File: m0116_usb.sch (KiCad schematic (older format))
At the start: 20 parts, among them J1 AVR-ISP-6, J2 USB_B_Mini, U1 ATmega32A-PU, Y1 16Mhz

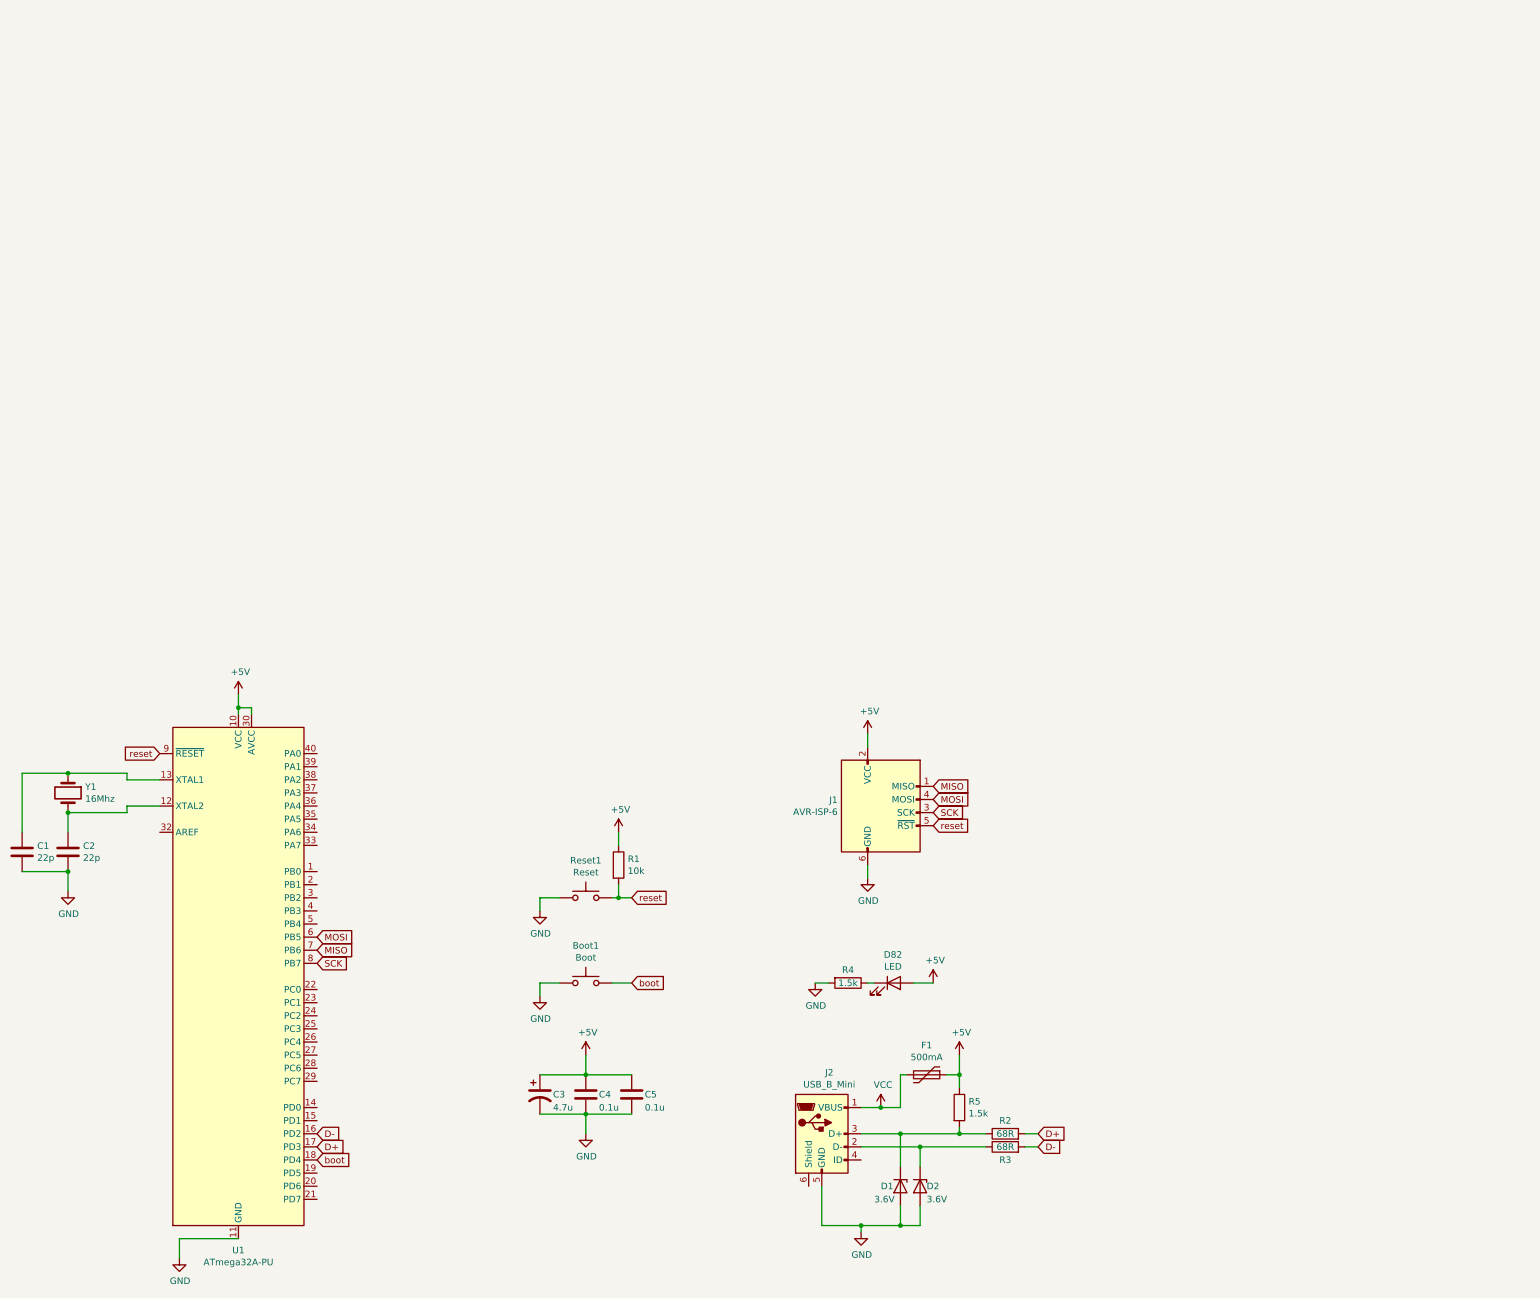
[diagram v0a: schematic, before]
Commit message: finished
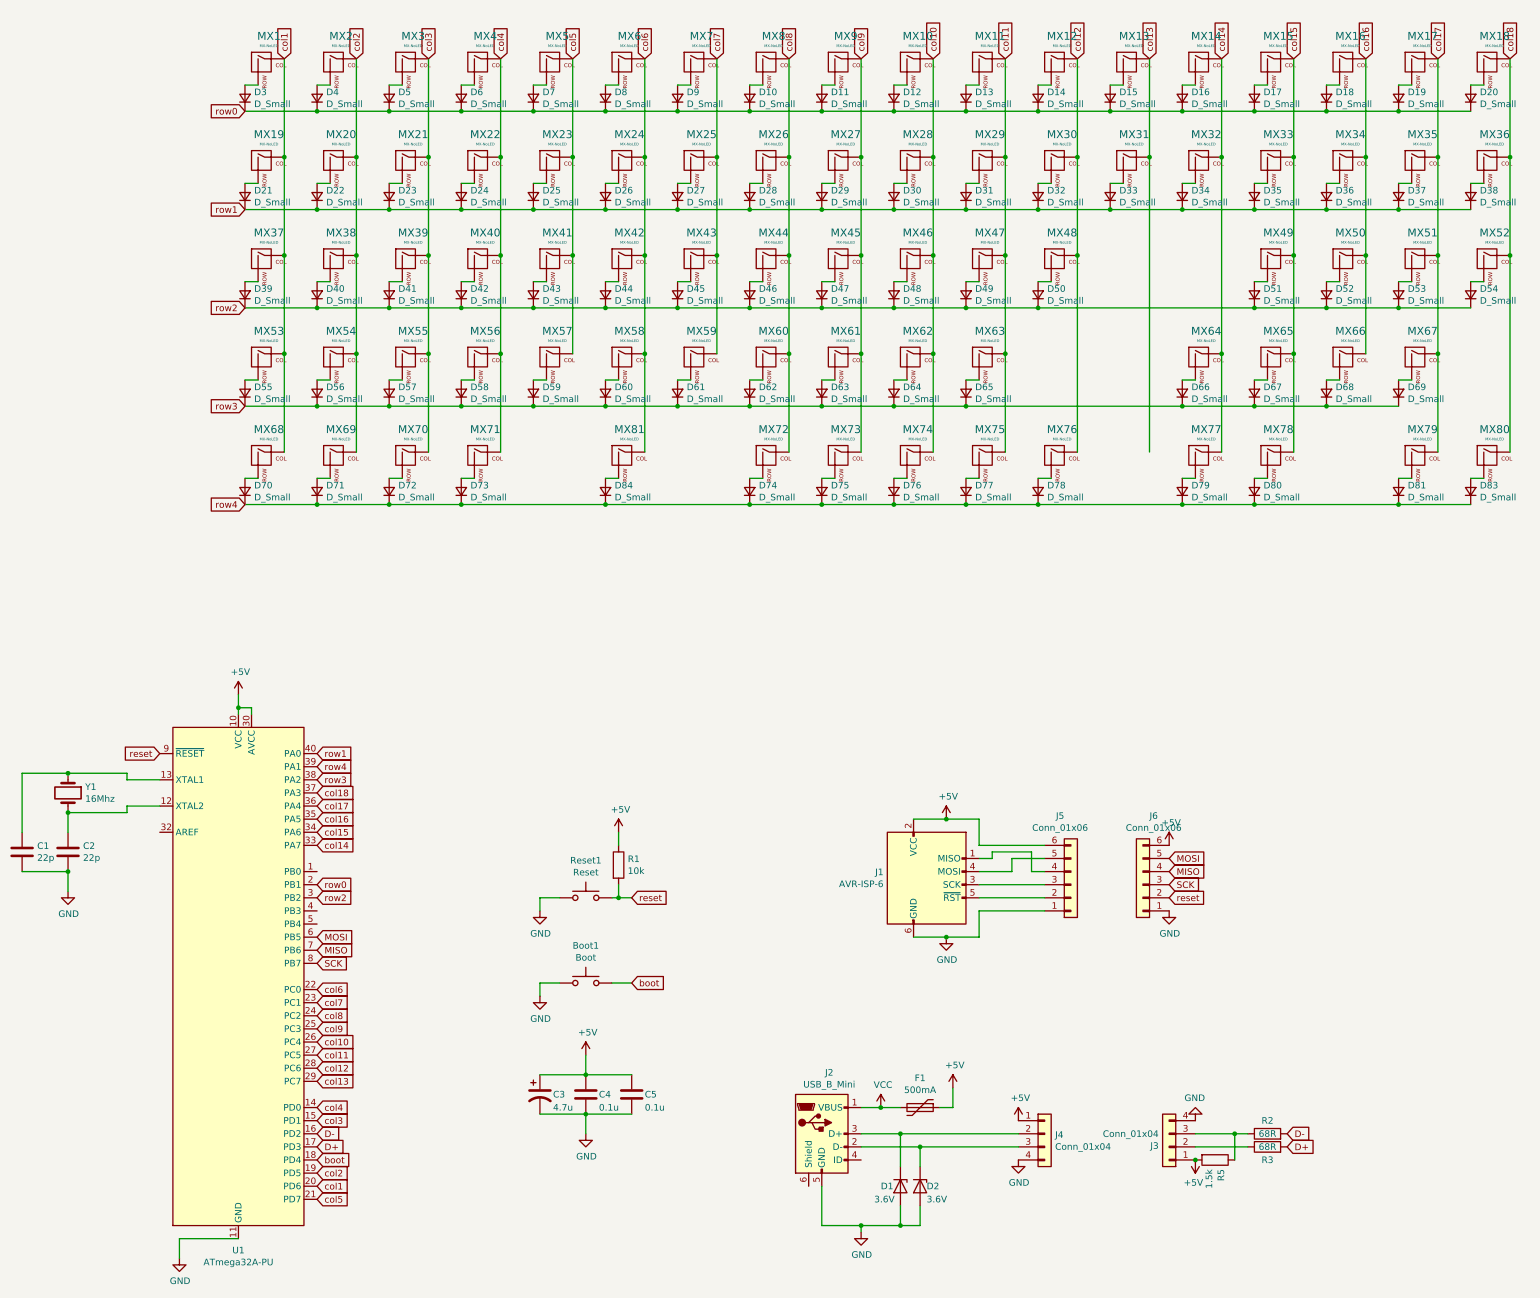
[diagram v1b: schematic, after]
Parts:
- removed D82: LED, LED_THT:LED_D3.0mm, symbol Device:LED
- removed R4: 1.5k, Resistor_THT:R_Axial_DIN0207_L6.3mm_D2.5mm_P10.16mm_Horizontal, symbol Device:R
- added D10, D11, D12, D13, D14, D15, D16, D17, D18, D19, D20, D21, D22, D23, D24, D25, D26, D27, D28, D29, D3, D30, D31, D32, D33, D34, D35, D36, D37, D38, D39, D4, D40, D41, D42, D43, D44, D45, D46, D47, D48, D49, D5, D50, D51, D52, D53, D54, D55, D56, D57, D58, D59, D6, D60, D61, D62, D63, D64, D65, D66, D67, D68, D69, D7, D70, D71, D72, D73, D74, D75, D76, D77, D78, D79, D8, D80, D81, D83, D84, D9: D_Small, Diode_THT:D_DO-35_SOD27_P7.62mm_Horizontal, symbol Device:D_Small
- added J3, J4: Conn_01x04, Connector_PinHeader_2.54mm:PinHeader_1x04_P2.54mm_Vertical, symbol Connector_Generic:Conn_01x04
- added J5, J6: Conn_01x06, Connector_PinHeader_2.54mm:PinHeader_1x06_P2.54mm_Vertical, symbol Connector_Generic:Conn_01x06
- added MX1, MX10, MX11, MX12, MX13, MX14, MX15, MX16, MX17, MX18, MX19, MX2, MX20, MX21, MX22, MX23, MX24, MX25, MX26, MX27, MX28, MX29, MX3, MX30, MX31, MX32, MX33, MX34, MX35, MX36, MX37, MX38, MX39, MX4, MX40, MX41, MX42, MX43, MX44, MX45, MX46, MX47, MX48, MX49, MX5, MX50, MX51, MX52, MX53, MX54, MX55, MX56, MX57, MX58, MX59, MX6, MX60, MX61, MX62, MX63, MX64, MX65, MX66, MX67, MX68, MX69, MX7, MX70, MX71, MX72, MX73, MX74, MX75, MX76, MX77, MX78, MX79, MX8, MX80, MX81, MX9: MX-NoLED, Alps_Only:ALPS-1U, symbol MX_Alps_Hybrid:MX-NoLED
- F1: footprint custom_parts:Fuse_Littelfuse_395Series -> Fuse:Fuse_Littelfuse_395Series
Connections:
- net +5V: now also R5.2, J3.1 (Pin_1), J4.1 (Pin_1), J5.6 (Pin_6), J6.6 (Pin_6); no longer R5.1
- net D+: now also R3.2; no longer R2.2
- net D-: now also R2.2; no longer R3.2
- net GND: now also J3.4 (Pin_4), J4.4 (Pin_4), J5.1 (Pin_1), J6.1 (Pin_1)
- net MISO: now also J6.4 (Pin_4); no longer J1.1 (MISO)
- net MOSI: now also J6.5 (Pin_5); no longer J1.4 (MOSI)
- net SCK: now also J6.3 (Pin_3); no longer J1.3 (SCK)
- net reset: now also J6.2 (Pin_2); no longer J1.5 (~RST)
- net col4: now reaches U1.14 (PD0)
- net col4: now also MX22.1 (COL), MX4.1 (COL), MX40.1 (COL), MX56.1 (COL), MX71.1 (COL)
- net col3: now reaches U1.15 (PD1)
- net col3: now also MX21.1 (COL), MX3.1 (COL), MX39.1 (COL), MX55.1 (COL), MX70.1 (COL)
- net col2: now reaches U1.19 (PD5)
- net col2: now also MX2.1 (COL), MX20.1 (COL), MX38.1 (COL), MX54.1 (COL), MX69.1 (COL)
- net row0: now reaches U1.2 (PB1)
- net row0: now also D10.1 (K), D11.1 (K), D12.1 (K), D13.1 (K), D14.1 (K), D15.1 (K), D16.1 (K), D17.1 (K), D18.1 (K), D19.1 (K), D20.1 (K), D3.1 (K), D4.1 (K), D5.1 (K), D6.1 (K), D7.1 (K), D8.1 (K), D9.1 (K)
- net col1: now reaches U1.20 (PD6)
- net col1: now also MX1.1 (COL), MX19.1 (COL), MX37.1 (COL), MX53.1 (COL), MX68.1 (COL)
- net col5: now reaches U1.21 (PD7)
- net col5: now also MX23.1 (COL), MX41.1 (COL), MX5.1 (COL), MX57.1 (COL)
- net col6: now reaches U1.22 (PC0)
- net col6: now also MX24.1 (COL), MX42.1 (COL), MX58.1 (COL), MX6.1 (COL), MX81.1 (COL)
- net col7: now reaches U1.23 (PC1)
- net col7: now also MX25.1 (COL), MX43.1 (COL), MX59.1 (COL), MX7.1 (COL)
- net col8: now reaches U1.24 (PC2)
- net col8: now also MX26.1 (COL), MX44.1 (COL), MX60.1 (COL), MX72.1 (COL), MX8.1 (COL)
- net col9: now reaches U1.25 (PC3)
- net col9: now also MX27.1 (COL), MX45.1 (COL), MX61.1 (COL), MX73.1 (COL), MX9.1 (COL)
- net col10: now reaches U1.26 (PC4)
- net col10: now also MX10.1 (COL), MX28.1 (COL), MX46.1 (COL), MX62.1 (COL), MX74.1 (COL)
- net col11: now reaches U1.27 (PC5)
- net col11: now also MX11.1 (COL), MX29.1 (COL), MX47.1 (COL), MX63.1 (COL), MX75.1 (COL)
- net col12: now reaches U1.28 (PC6)
- net col12: now also MX12.1 (COL), MX30.1 (COL), MX48.1 (COL), MX76.1 (COL)
- net col13: now reaches U1.29 (PC7)
- net col13: now also MX13.1 (COL), MX31.1 (COL)
- net row2: now reaches U1.3 (PB2)
- net row2: now also D39.1 (K), D40.1 (K), D41.1 (K), D42.1 (K), D43.1 (K), D44.1 (K), D45.1 (K), D46.1 (K), D47.1 (K), D48.1 (K), D49.1 (K), D50.1 (K), D51.1 (K), D52.1 (K), D53.1 (K), D54.1 (K)
- net col14: now reaches U1.33 (PA7)
- net col14: now also MX14.1 (COL), MX32.1 (COL), MX64.1 (COL), MX77.1 (COL)
- net col15: now reaches U1.34 (PA6)
- net col15: now also MX15.1 (COL), MX33.1 (COL), MX49.1 (COL), MX65.1 (COL), MX78.1 (COL)
- net col16: now reaches U1.35 (PA5)
- net col16: now also MX16.1 (COL), MX34.1 (COL), MX50.1 (COL), MX66.1 (COL)
- net col17: now reaches U1.36 (PA4)
- net col17: now also MX17.1 (COL), MX35.1 (COL), MX51.1 (COL), MX67.1 (COL), MX79.1 (COL)
- net col18: now reaches U1.37 (PA3)
- net col18: now also MX18.1 (COL), MX36.1 (COL), MX52.1 (COL), MX80.1 (COL)
- net row3: now reaches U1.38 (PA2)
- net row3: now also D55.1 (K), D56.1 (K), D57.1 (K), D58.1 (K), D59.1 (K), D60.1 (K), D61.1 (K), D62.1 (K), D63.1 (K), D64.1 (K), D65.1 (K), D66.1 (K), D67.1 (K), D68.1 (K), D69.1 (K)
- net row4: now reaches U1.39 (PA1)
- net row4: now also D70.1 (K), D71.1 (K), D72.1 (K), D73.1 (K), D74.1 (K), D75.1 (K), D76.1 (K), D77.1 (K), D78.1 (K), D79.1 (K), D80.1 (K), D81.1 (K), D83.1 (K), D84.1 (K)
- net row1: now reaches U1.40 (PA0)
- net row1: now also D21.1 (K), D22.1 (K), D23.1 (K), D24.1 (K), D25.1 (K), D26.1 (K), D27.1 (K), D28.1 (K), D29.1 (K), D30.1 (K), D31.1 (K), D32.1 (K), D33.1 (K), D34.1 (K), D35.1 (K), D36.1 (K), D37.1 (K), D38.1 (K)
- net at D2.1 (K), J2.2 (D-): now also J4.3 (Pin_3); no longer R3.1
- net at D1.1 (K), J2.3 (D+): now also J4.2 (Pin_2); no longer R2.1, R5.2
- new net: J3.2 (Pin_2), R3.1
- new net: J3.3 (Pin_3), R2.1, R5.1
- new net: D3.2 (A), MX1.2 (ROW)
- new net: D4.2 (A), MX2.2 (ROW)
- new net: D5.2 (A), MX3.2 (ROW)
- new net: D6.2 (A), MX4.2 (ROW)
- new net: D7.2 (A), MX5.2 (ROW)
- new net: D8.2 (A), MX6.2 (ROW)
- new net: D9.2 (A), MX7.2 (ROW)
- new net: D10.2 (A), MX8.2 (ROW)
- new net: D11.2 (A), MX9.2 (ROW)
- new net: D12.2 (A), MX10.2 (ROW)
- new net: D13.2 (A), MX11.2 (ROW)
- new net: D14.2 (A), MX12.2 (ROW)
- new net: D15.2 (A), MX13.2 (ROW)
- new net: D16.2 (A), MX14.2 (ROW)
- new net: D17.2 (A), MX15.2 (ROW)
- new net: D18.2 (A), MX16.2 (ROW)
- new net: D19.2 (A), MX17.2 (ROW)
- new net: D20.2 (A), MX18.2 (ROW)
- new net: D21.2 (A), MX19.2 (ROW)
- new net: D22.2 (A), MX20.2 (ROW)
- new net: D23.2 (A), MX21.2 (ROW)
- new net: D24.2 (A), MX22.2 (ROW)
- new net: D25.2 (A), MX23.2 (ROW)
- new net: D26.2 (A), MX24.2 (ROW)
- new net: D27.2 (A), MX25.2 (ROW)
- new net: D28.2 (A), MX26.2 (ROW)
- new net: D29.2 (A), MX27.2 (ROW)
- new net: D30.2 (A), MX28.2 (ROW)
- new net: D31.2 (A), MX29.2 (ROW)
- new net: D32.2 (A), MX30.2 (ROW)
- new net: D33.2 (A), MX31.2 (ROW)
- new net: D34.2 (A), MX32.2 (ROW)
- new net: D35.2 (A), MX33.2 (ROW)
- new net: D36.2 (A), MX34.2 (ROW)
- new net: D37.2 (A), MX35.2 (ROW)
- new net: D38.2 (A), MX36.2 (ROW)
- new net: D39.2 (A), MX37.2 (ROW)
- new net: D40.2 (A), MX38.2 (ROW)
- new net: D41.2 (A), MX39.2 (ROW)
- new net: D42.2 (A), MX40.2 (ROW)
- new net: D43.2 (A), MX41.2 (ROW)
- new net: D44.2 (A), MX42.2 (ROW)
- new net: D45.2 (A), MX43.2 (ROW)
- new net: D46.2 (A), MX44.2 (ROW)
- new net: D47.2 (A), MX45.2 (ROW)
- new net: D48.2 (A), MX46.2 (ROW)
- new net: D49.2 (A), MX47.2 (ROW)
- new net: D50.2 (A), MX48.2 (ROW)
- new net: D51.2 (A), MX49.2 (ROW)
- new net: D52.2 (A), MX50.2 (ROW)
- new net: D53.2 (A), MX51.2 (ROW)
- new net: D54.2 (A), MX52.2 (ROW)
- new net: D55.2 (A), MX53.2 (ROW)
- new net: D56.2 (A), MX54.2 (ROW)
- new net: D57.2 (A), MX55.2 (ROW)
- new net: D58.2 (A), MX56.2 (ROW)
- new net: D59.2 (A), MX57.2 (ROW)
- new net: D60.2 (A), MX58.2 (ROW)
- new net: D61.2 (A), MX59.2 (ROW)
- new net: D62.2 (A), MX60.2 (ROW)
- new net: D63.2 (A), MX61.2 (ROW)
- new net: D64.2 (A), MX62.2 (ROW)
- new net: D65.2 (A), MX63.2 (ROW)
- new net: D66.2 (A), MX64.2 (ROW)
- new net: D67.2 (A), MX65.2 (ROW)
- new net: D68.2 (A), MX66.2 (ROW)
- new net: D69.2 (A), MX67.2 (ROW)
- new net: D70.2 (A), MX68.2 (ROW)
- new net: D71.2 (A), MX69.2 (ROW)
- new net: D72.2 (A), MX70.2 (ROW)
- new net: D73.2 (A), MX71.2 (ROW)
- new net: D74.2 (A), MX72.2 (ROW)
- new net: D75.2 (A), MX73.2 (ROW)
- new net: D76.2 (A), MX74.2 (ROW)
- new net: D77.2 (A), MX75.2 (ROW)
- new net: D78.2 (A), MX76.2 (ROW)
- new net: D79.2 (A), MX77.2 (ROW)
- new net: D80.2 (A), MX78.2 (ROW)
- new net: D81.2 (A), MX79.2 (ROW)
- new net: D83.2 (A), MX80.2 (ROW)
- new net: D84.2 (A), MX81.2 (ROW)
- new net: J1.1 (MISO), J5.4 (Pin_4)
- new net: J1.3 (SCK), J5.3 (Pin_3)
- new net: J1.4 (MOSI), J5.5 (Pin_5)
- new net: J1.5 (~RST), J5.2 (Pin_2)
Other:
- moved on the sheet: F1, R2, R3, R5
